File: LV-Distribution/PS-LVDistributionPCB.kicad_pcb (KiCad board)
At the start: 2 copper layers, 150.7 x 65 mm, 48 parts, among them J1 Conn_01x02, J10 Conn_01x02, J11 Conn_01x02, J12 Conn_01x02, J13 Conn_01x02, J14 Conn_01x02, J17 MX150_02x10_RightAngle, J2 Conn_01x02, J3 Conn_01x02, J4 Conn_01x02, J5 Conn_01x02, J6 Conn_01x02, J7 Conn_01x02, J8 Conn_01x02, J9 Conn_01x02

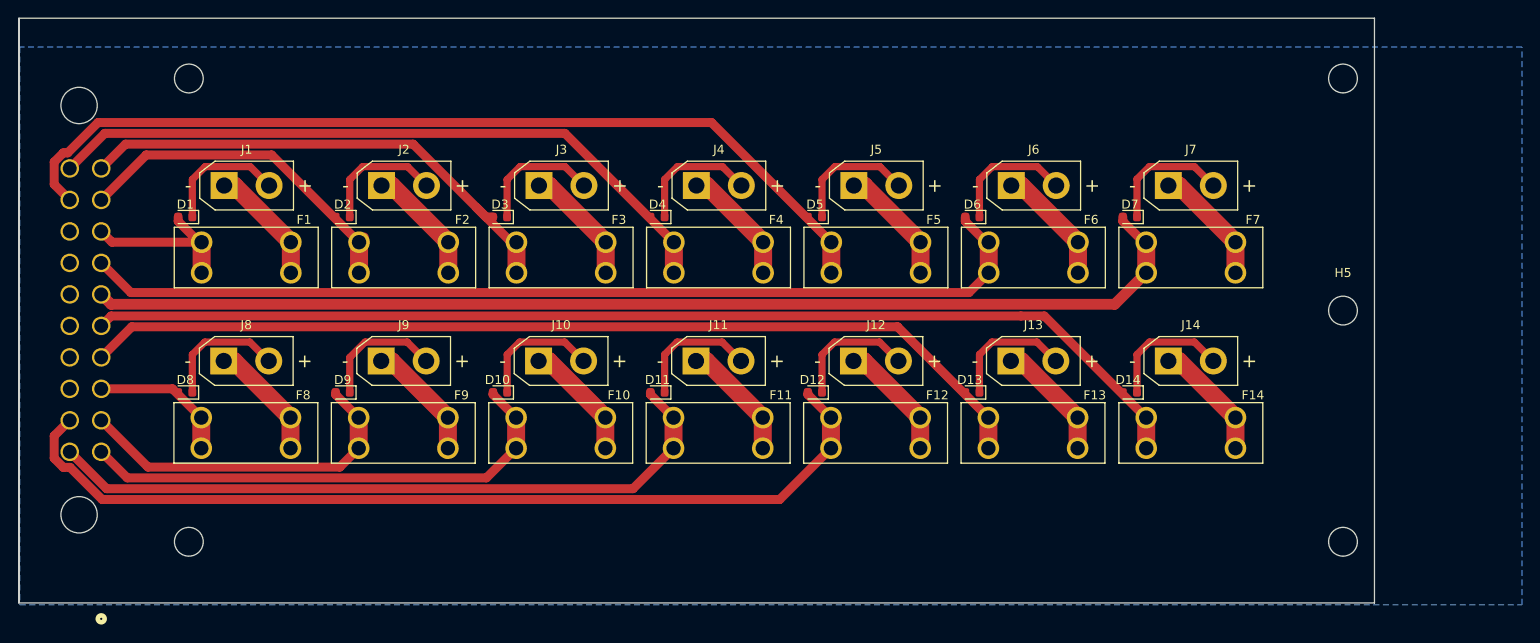
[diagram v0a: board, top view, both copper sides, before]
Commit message: fixed 3d + gerbers
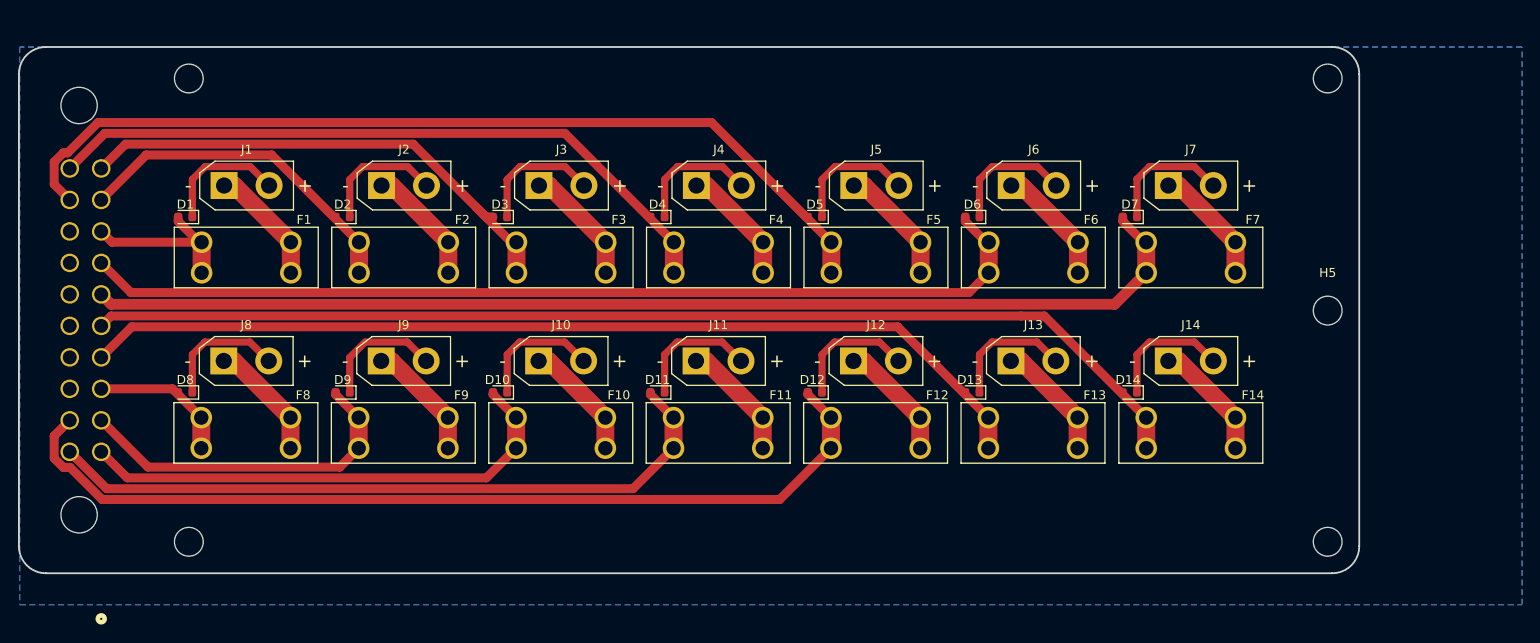
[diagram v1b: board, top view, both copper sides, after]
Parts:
- moved H2 1.70 mm to (231.4, 61.5)
- moved H4 1.70 mm to (231.4, 113.0)
- moved H5 1.70 mm to (231.4, 87.3)
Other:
- board size 150.7 x 65 mm -> 149 x 58.5 mm
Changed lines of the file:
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@@
 	(footprint "MountingHole:MountingHole_3.2mm_M3"
 		(layer "F.Cu")
-		(at 233.1 87.3)
+		(at 231.4 87.3)
 		(descr "Mounting Hole 3.2mm, no annular, M3")
 		(tags "mounting hole 3.2mm no annular m3")
@@
 	(footprint "MountingHole:MountingHole_3.2mm_M3"
 		(layer "F.Cu")
-		(at 233.1 61.5)
+		(at 231.4 61.5)
 		(descr "Mounting Hole 3.2mm, no annular, M3")
 		(tags "mounting hole 3.2mm no annular m3")
@@
 	(footprint "MountingHole:MountingHole_3.2mm_M3"
 		(layer "F.Cu")
-		(at 233.1 113)
+		(at 231.4 113)
 		(descr "Mounting Hole 3.2mm, no annular, M3")
 		(tags "mounting hole 3.2mm no annular m3")
@@
 		)
 		(fp_line
+			(start -16.660395 -9.152805)
+			(end 48.160405 -9.152805)
+			(stroke
+				(width 0.0254)
+				(type solid)
+			)
+			(layer "B.SilkS")
+		)
+		(fp_line
 			(start 48.287405 -8.845255)
 			(end 48.287405 0.677)
@@
 		)
 		(fp_line
-			(start -16.660395 -9.152805)
-			(end 48.160405 -9.152805)
-			(stroke
-				(width 0.0254)
-				(type solid)
-			)
-			(layer "Edge.Cuts")
-		)
-		(fp_line
 			(start 48.414405 -42.274404)
 			(end 48.414405 1.282701)
@@
 				(name "0348302001.stp")
 				(type model)
-				(checksum "9310518C80B9A11C3C709B68A6EC8CDD")
+				(checksum "03A4D46CEC60E7FBAAF483EA678A442B")
 			)
 		)
 		(model "kicad-embed://0348302001.stp"
 			(offset
-				(xyz -2.25 -8 -3)
+				(xyz -2.25 -8 -2.5)
 			)
 			(scale
@@
 		)
 	)
-	(gr_rect
-		(start 85.9 54.8)
-		(end 236.6 119.8)
+	(gr_line
+		(start 88.907196 58)
+		(end 231.907196 58)
+		(stroke
+			(width 0.2)
+			(type default)
+		)
+		(layer "Edge.Cuts")
+	)
+	(gr_line
+		(start 234.907196 61)
+		(end 234.907196 113.5)
+		(stroke
+			(width 0.2)
+			(type default)
+		)
+		(layer "Edge.Cuts")
+	)
+	(gr_line
+		(start 231.907196 116.5)
+		(end 88.907196 116.5)
+		(stroke
+			(width 0.2)
+			(type default)
+		)
+		(layer "Edge.Cuts")
+	)
+	(gr_arc
+		(start 234.907196 113.5)
+		(mid 234.028516 115.621319)
+		(end 231.907196 116.5)
+		(stroke
+			(width 0.2)
+			(type default)
+		)
+		(layer "Edge.Cuts")
+	)
+	(gr_arc
+		(start 231.907196 58)
+		(mid 234.028519 58.878678)
+		(end 234.907196 61)
+		(stroke
+			(width 0.2)
+			(type default)
+		)
+		(layer "Edge.Cuts")
+	)
+	(gr_line
+		(start 85.907196 113.5)
+		(end 85.907196 61)
+		(stroke
+			(width 0.2)
+			(type default)
+		)
+		(layer "Edge.Cuts")
+	)
+	(gr_arc
+		(start 85.907196 61)
+		(mid 86.785876 58.87868)
+		(end 88.907196 58)
+		(stroke
+			(width 0.2)
+			(type default)
+		)
+		(layer "Edge.Cuts")
+	)
+	(gr_arc
+		(start 88.907196 116.5)
+		(mid 86.785878 115.621319)
+		(end 85.907196 113.5)
 		(stroke
-			(width 0.05)
+			(width 0.2)
 			(type default)
 		)
-		(fill no)
 		(layer "Edge.Cuts")
 	)
